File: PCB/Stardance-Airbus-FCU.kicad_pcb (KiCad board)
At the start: 2 copper layers, 150.5 x 68.5 mm, 11 parts, among them SW1 SW_Push_45deg, SW10 SW_Push_45deg, SW2 SW_Push_45deg, SW3 SW_Push_45deg, SW4 SW_Push_45deg, SW5 RotaryEncoder_Switch, SW6 RotaryEncoder_Switch, SW7 RotaryEncoder_Switch, SW8 RotaryEncoder_Switch, SW9 SW_Push_45deg

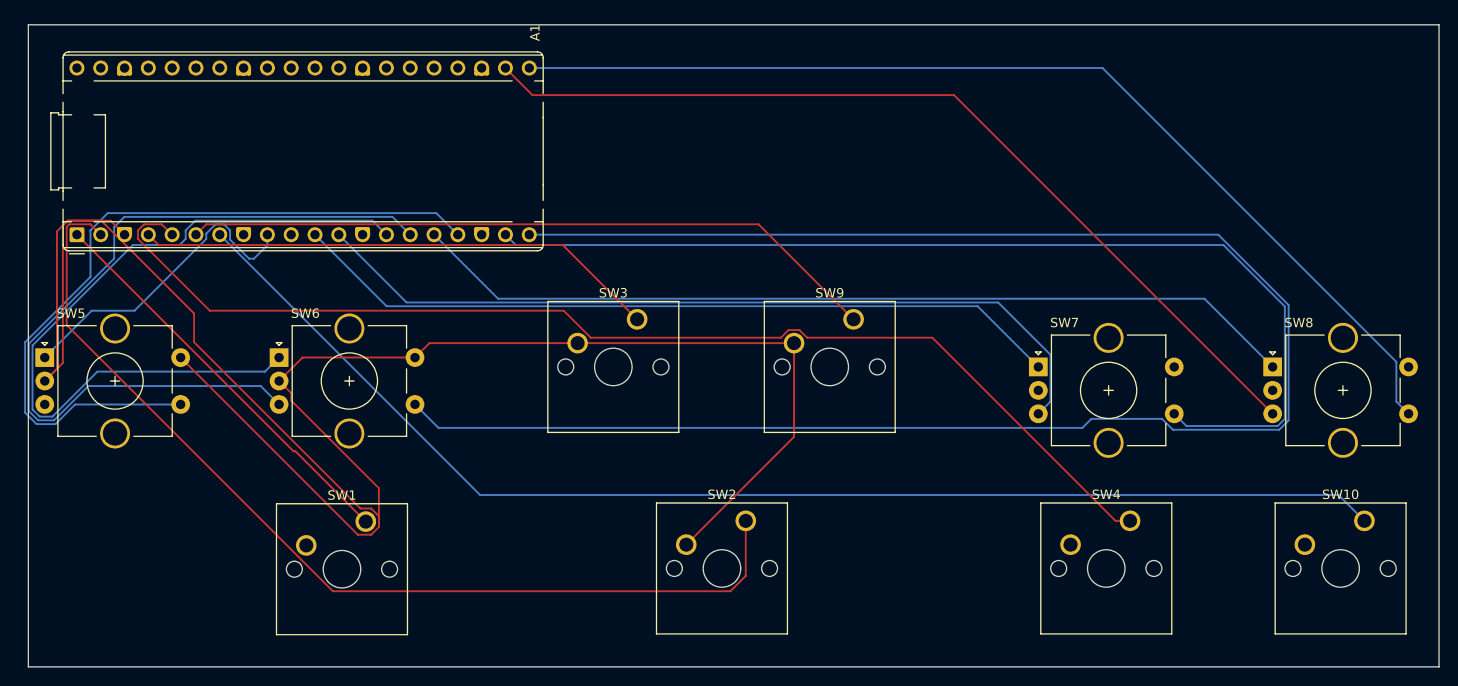
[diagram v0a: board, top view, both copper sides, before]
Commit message: revision 1 file uploads
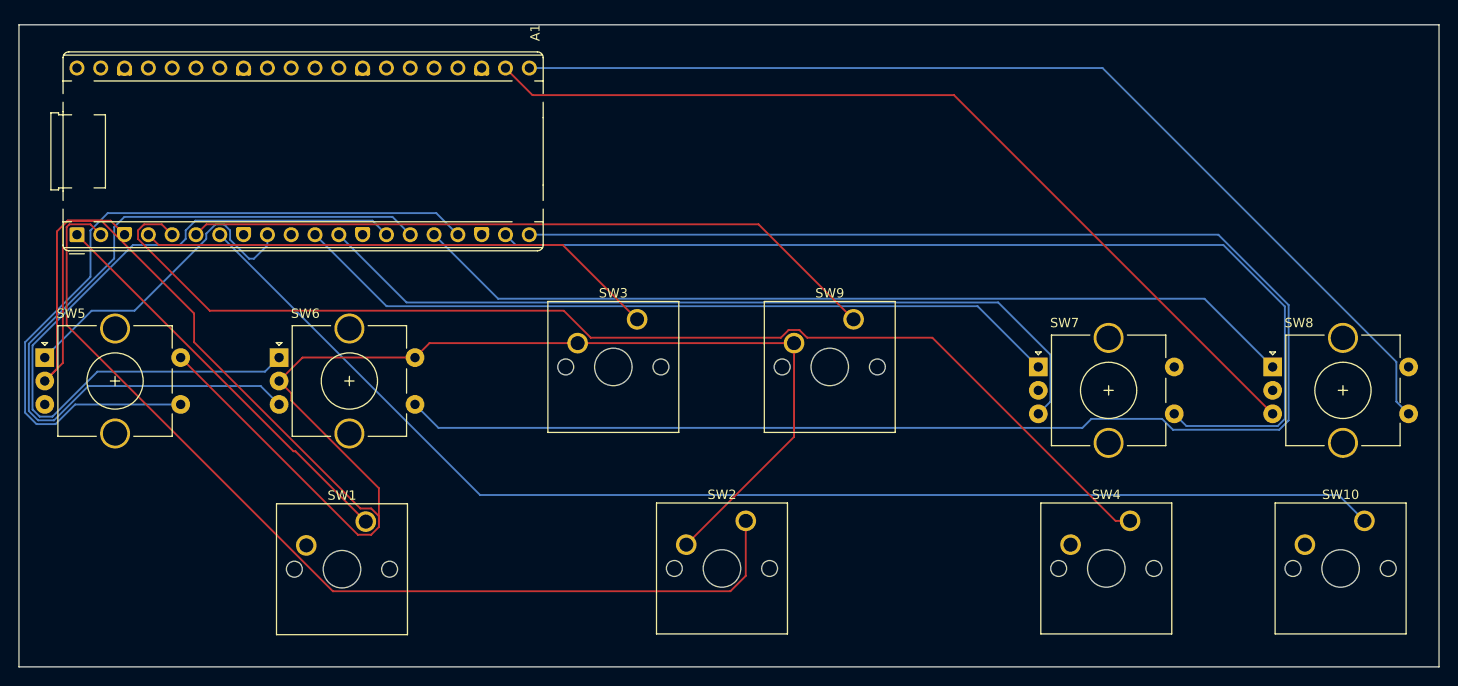
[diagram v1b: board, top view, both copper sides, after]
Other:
- board size 150.5 x 68.5 mm -> 151.5 x 68.5 mm
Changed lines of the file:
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@@
 			(outputformat 1)
 			(mirror no)
-			(drillshape 1)
+			(drillshape 0)
 			(scaleselection 1)
-			(outputdirectory "")
+			(outputdirectory "Gerbers/")
 		)
 	)
@@
 	)
 	(gr_rect
-		(start 57 32.5)
+		(start 56 32.5)
 		(end 207.5 101)
 		(stroke
